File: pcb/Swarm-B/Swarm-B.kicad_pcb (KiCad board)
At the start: 2 copper layers, 71.9 x 71.9 mm, 26 parts, among them J1 RX_Break, J2 5v_3Pi, J3 GND_3Pi, J4 I2C_3Pi, SW1 Bttn, U1 74LS32, U2 TSDP34138

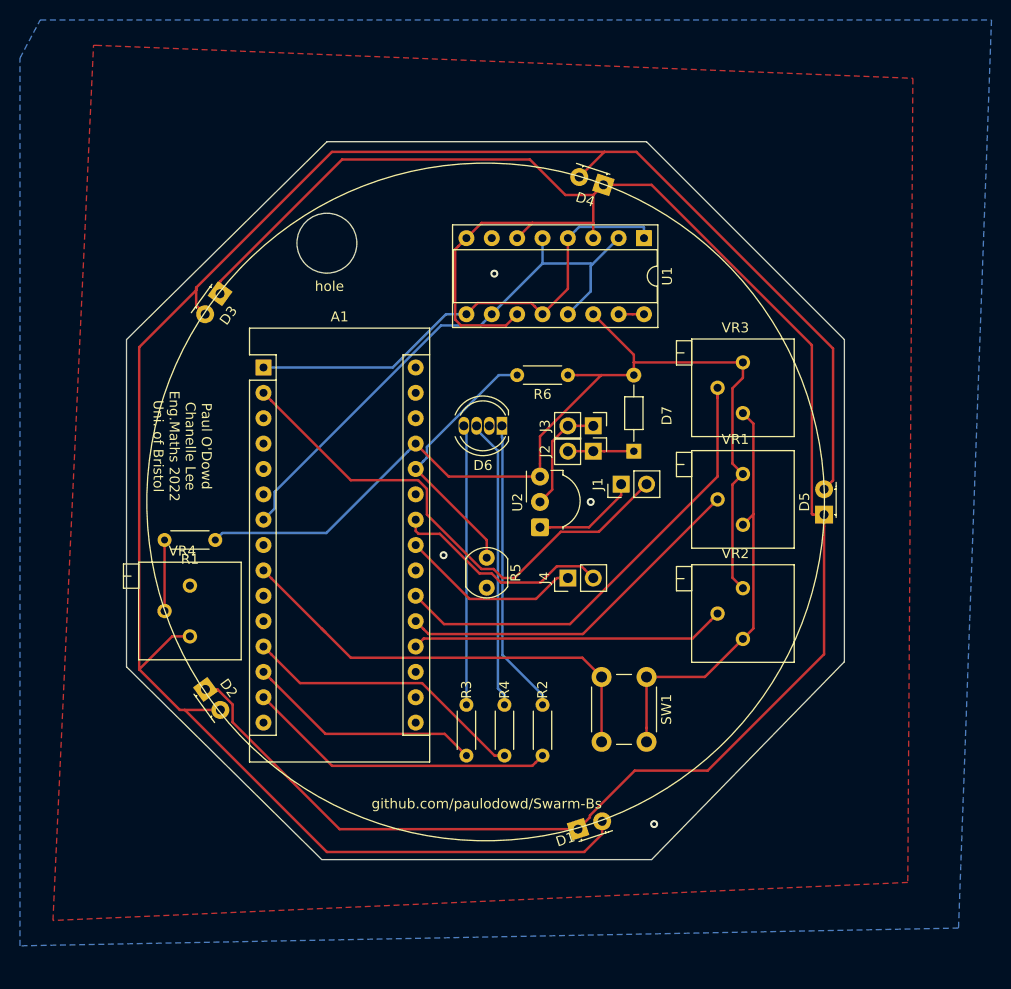
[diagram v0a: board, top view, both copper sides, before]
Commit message: update
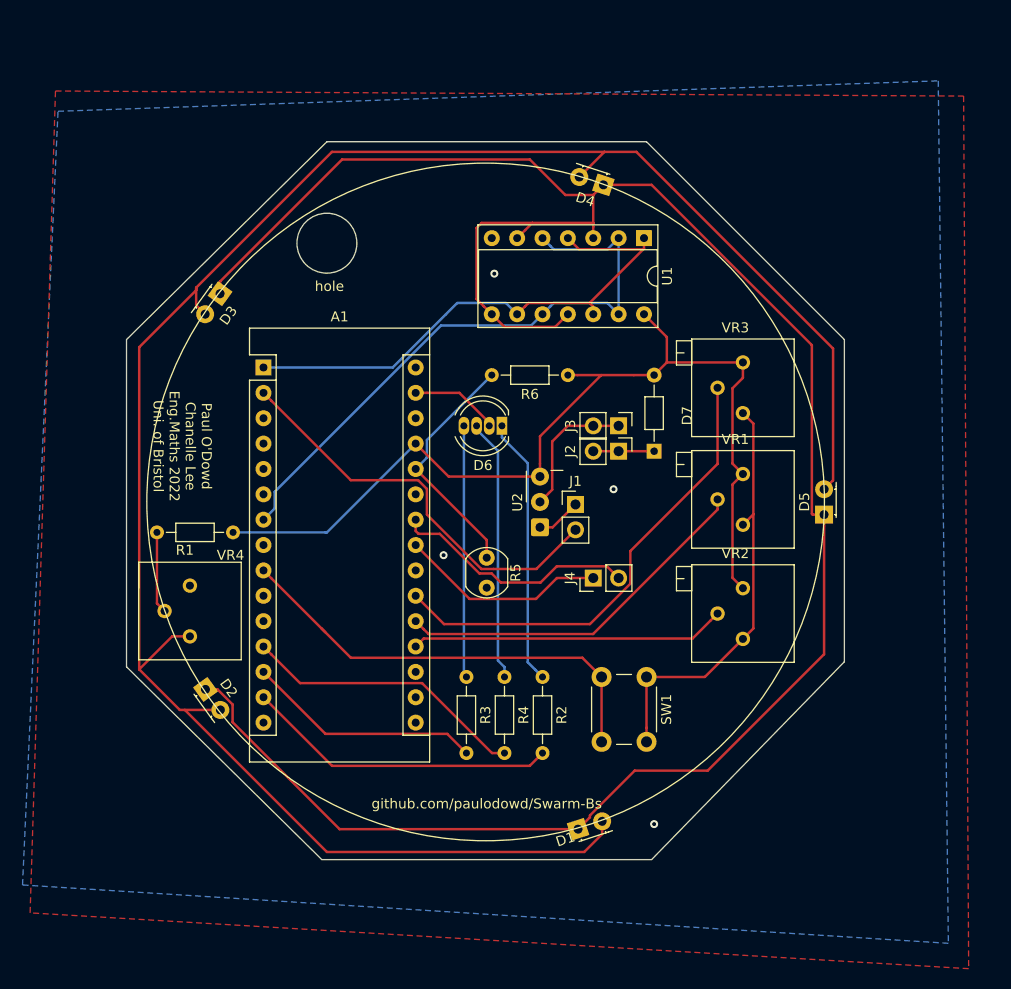
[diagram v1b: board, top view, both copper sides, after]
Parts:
- R1, R2, R3, R4, R6: footprint Resistor_THT:R_Axial_DIN0204_L3.6mm_D1.6mm_P5.08mm_Horizontal -> Resistor_THT:R_Axial_DIN0204_L3.6mm_D1.6mm_P7.62mm_Horizontal
- U1: footprint Package_DIP:DIP-16_W7.62mm_Socket -> Package_DIP:DIP-14_W7.62mm_Socket
- moved J1 5.00 mm to (127.8, 94.5), turned to 0 degrees
- moved R2 2.79 mm to (124.5, 111.8)
- moved R3 2.79 mm to (116.8, 111.8)
- moved R4 2.79 mm to (120.7, 111.8)
- moved J2 2.54 mm to (132.1, 89.2)
- moved J3 2.54 mm to (132.1, 86.6)
- moved J4 2.54 mm to (129.5, 101.9)
- moved D7 2.03 mm to (135.6, 89.2)
- moved R1 1.93 mm to (93.5, 97.3)
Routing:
- net GND: track 54.0 -> 65.5 mm
- net Net-(A1-Pad2): track 51.4 -> 41.7 mm
- net Net-(J1-Pad1): track 11.6 -> 5.58 mm
- net Net-(A1-Pad1): track 48.9 -> 54.4 mm
- net Net-(A1-Pad7): track 56.8 -> 62.2 mm
- net +5V: track 100.2 -> 96.6 mm
- net Net-(D6-Pad1): track 29.6 -> 26.8 mm
- net Net-(D6-Pad3): track 29.1 -> 26.4 mm
- net Net-(A1-Pad24): track 22.2 -> 24.7 mm
- net Net-(A1-Pad23): track 18.3 -> 20.9 mm
- net (no net): track 2.54 -> 0.00 mm
- net Net-(D6-Pad4): track 28.0 -> 25.6 mm
- net Net-(A1-Pad26): track 26.5 -> 24.4 mm
- net Net-(R1-Pad2): track 7.11 -> 8.19 mm
- net Net-(D1-Pad1): track 217.7 -> 218.7 mm
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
